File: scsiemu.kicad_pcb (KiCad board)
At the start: 2 copper layers, 65 x 41.7 mm, 38 parts, among them J1 RasPi, J2 SCSI, J3 USB_POWER, J4 POWER 5V, J5 I2C, U1 74LS641-1, U2 74LS641-1, U3 74LS641-1, U4 74LS641-1

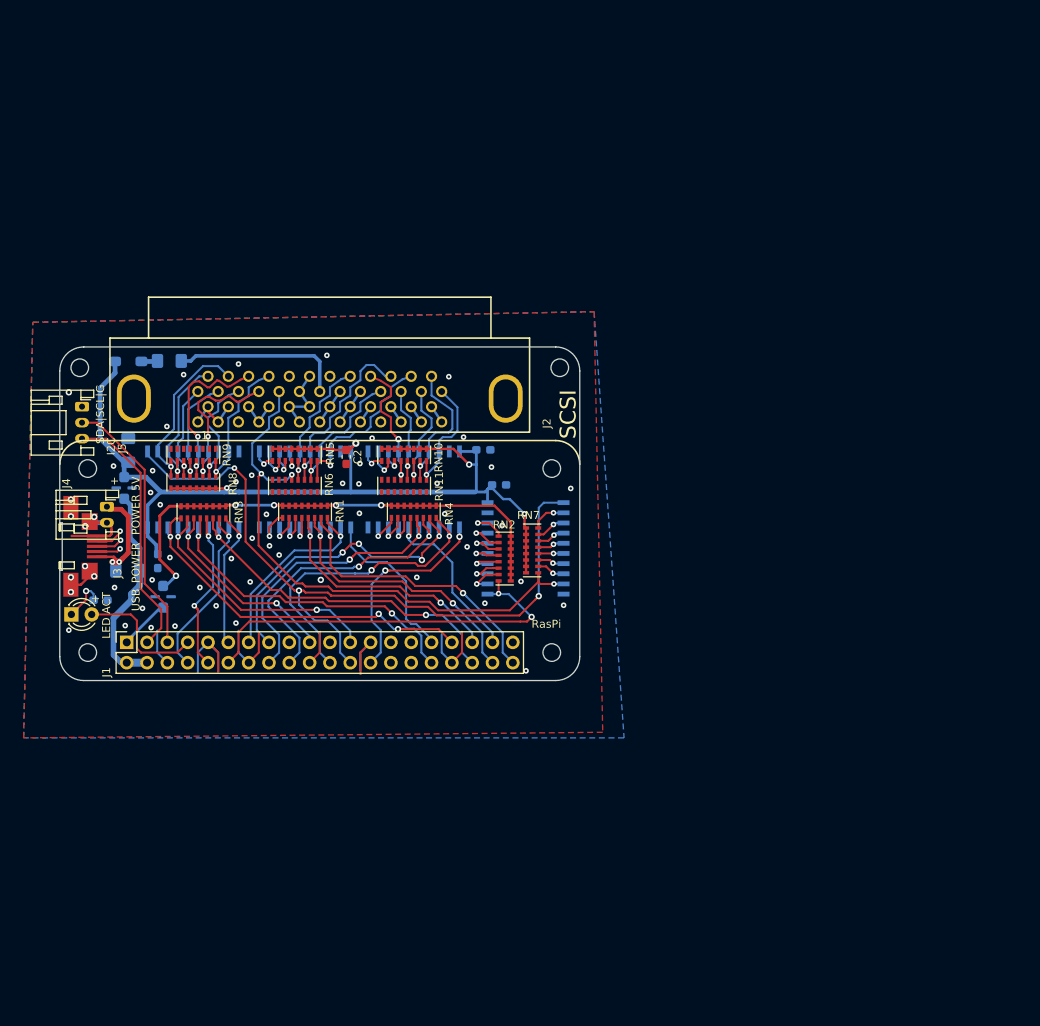
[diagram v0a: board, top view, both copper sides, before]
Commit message: update libs update PCBs update schematic
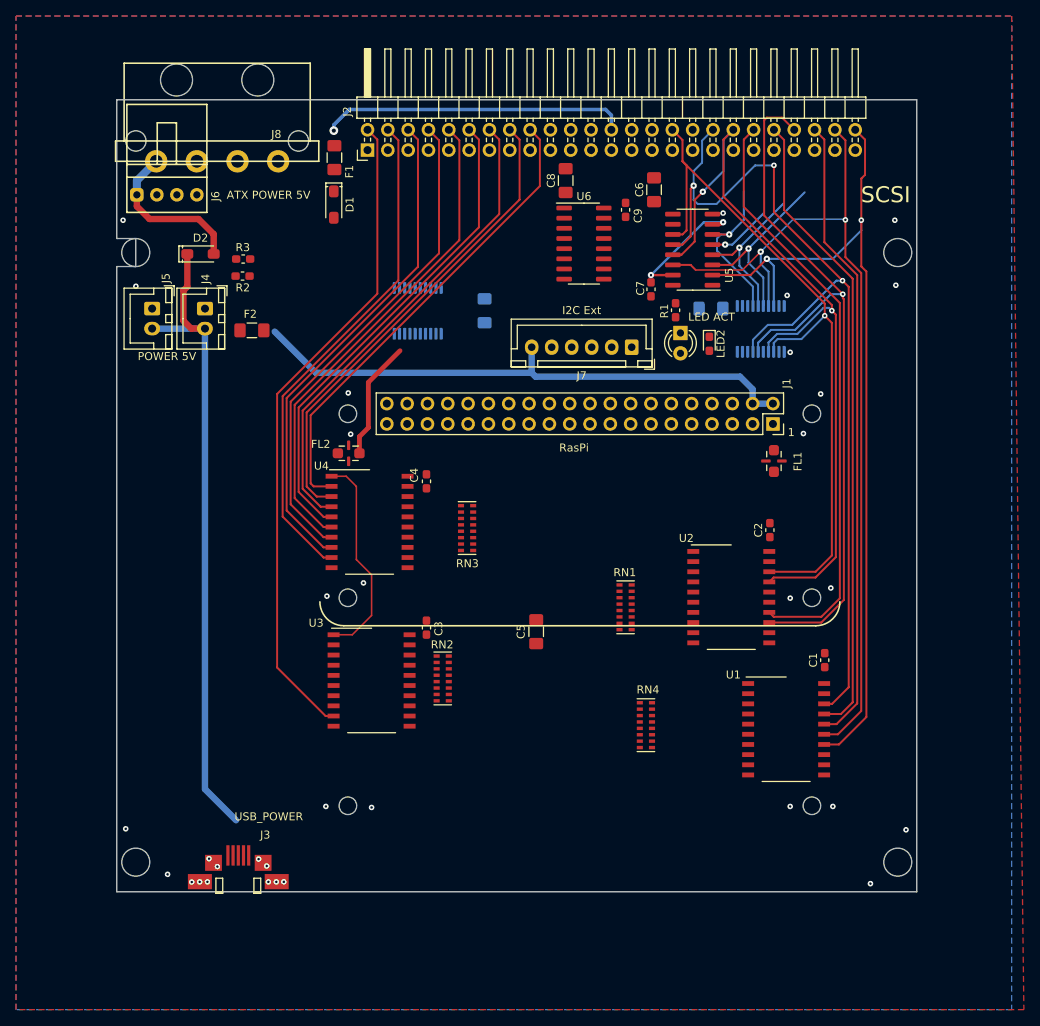
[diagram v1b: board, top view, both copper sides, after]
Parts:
- removed REF** (x6): MountingHole_2.2mm_M2, MountingHole:MountingHole_2.2mm_M2
- removed RN10, RN5, RN7, RN8: 220, Resistor_SMD:R_Cat16-8
- removed RN11, RN6, RN9: 330, Resistor_SMD:R_Cat16-8
- added C10: 10u, Capacitor_SMD:C_1206_3216Metric_Pad1.42x1.75mm_HandSolder, B.Cu at (183.9, 64.0)
- added C11: 10u, Capacitor_SMD:C_1206_3216Metric_Pad1.42x1.75mm_HandSolder, B.Cu at (155.6, 64.3)
- added C6: 10u, Capacitor_SMD:C_1206_3216Metric_Pad1.42x1.75mm_HandSolder, F.Cu at (176.8, 49.1)
- added C7: 2.2u, Capacitor_SMD:C_0603_1608Metric_Pad1.05x0.95mm_HandSolder, F.Cu at (176.4, 61.6)
- added C8: 10u, Capacitor_SMD:C_1206_3216Metric_Pad1.42x1.75mm_HandSolder, F.Cu at (165.7, 48.0)
- added C9: 2.2u, Capacitor_SMD:C_0603_1608Metric_Pad1.05x0.95mm_HandSolder, F.Cu at (173.2, 51.7)
- added D2: SBD, local_lib:D_SOD-123_HandSoldering, F.Cu at (120.1, 57.2)
- added J6: AT Power 5V (171826-4), local_lib:Molex_171826-4, F.Cu at (119.6, 49.8)
- added J7: I2C Ext, Connector_JST:JST_XH_B6B-XH-A_1x06_P2.50mm_Vertical, F.Cu at (174.0, 68.8)
- added J8: AT Power 5V (641737-1), local_lib:TE_641737-1, F.Cu at (122.2, 35.4)
- added LED2: LED ACT, LED_SMD:LED_0603_1608Metric_Pad1.05x0.95mm_HandSolder, F.Cu at (183.7, 68.4)
- added MH1: Raspi Mount, MountingHole:MountingHole_2.2mm_M2, F.Cu at (138.5, 100.2)
- added MH10: Raspi Mount, MountingHole:MountingHole_2.2mm_M2, F.Cu at (138.5, 126.2)
- added MH2: Raspi Mount, MountingHole:MountingHole_2.2mm_M2, F.Cu at (138.5, 77.2)
- added MH3: Raspi Mount, MountingHole:MountingHole_2.2mm_M2, F.Cu at (196.5, 77.2)
- added MH4: Raspi Mount, MountingHole:MountingHole_2.2mm_M2, F.Cu at (196.5, 100.2)
- added MH5: HDD Mount, MountingHole:MountingHole_3.5mm, F.Cu at (112.0, 57.0)
- added MH6: HDD Mount, MountingHole:MountingHole_3.5mm, F.Cu at (112.0, 133.2)
- added MH7: HDD Mount, MountingHole:MountingHole_3.5mm, F.Cu at (207.2, 57.0)
- added MH8: HDD Mount, MountingHole:MountingHole_3.5mm, F.Cu at (207.2, 133.2)
- added MH9: Raspi Mount, MountingHole:MountingHole_2.2mm_M2, F.Cu at (196.5, 126.2)
- added R2: 2.2k, Resistor_SMD:R_0603_1608Metric_Pad1.05x0.95mm_HandSolder, F.Cu at (125.3, 59.9)
- added R3: 2.7k, Resistor_SMD:R_0603_1608Metric_Pad1.05x0.95mm_HandSolder, F.Cu at (125.4, 57.8)
- added U5: DS2105Z, Package_SO:SOIC-16_3.9x9.9mm_P1.27mm, F.Cu at (181.6, 56.6)
- added U6: DS2105Z, Package_SO:SOIC-16_3.9x9.9mm_P1.27mm, F.Cu at (168.0, 55.9)
- added U7: TL2218-285, Package_SO:TSSOP-20_4.4x6.5mm_P0.65mm, B.Cu at (190.1, 66.5)
- added U8: TL2218-285, Package_SO:TSSOP-20_4.4x6.5mm_P0.65mm, B.Cu at (147.2, 64.3)
- C1, C4: value 0.1u JB -> 0.1u; moved to F.Cu
- C2: value 0.1u JB -> 0.1u
- C3: value 0.1u JIS B -> 0.1u; moved to F.Cu
- C5: value 10u JB -> 10u; moved to F.Cu
- D1: footprint cd_device:D_SOD-123_HandSoldering -> local_lib:D_SOD-123_HandSoldering; moved to F.Cu
- F1, FL1, FL2, R1, U1, U2, U3, U4: moved to F.Cu
- F2: value 1A -> 2A; moved to F.Cu
- J2: footprint local_lib:DSUB50P -> Connector_PinHeader_2.54mm:PinHeader_2x25_P2.54mm_Horizontal
- J4: footprint Connector_JST:JST_PH_S2B-PH-K_1x02_P2.00mm_Horizontal -> Connector_JST:JST_XH_B2B-XH-A_1x02_P2.50mm_Vertical
- J5: value I2C -> POWER 5V; footprint Connector_JST:JST_PH_S3B-PH-K_1x03_P2.00mm_Horizontal -> Connector_JST:JST_XH_B2B-XH-A_1x02_P2.50mm_Vertical
- moved J1 85.3 mm to (191.6, 78.4), turned to 270 degrees
- moved LED1 83.9 mm to (180.1, 67.1), turned to 270 degrees
- moved R1 80.5 mm to (179.5, 64.2), turned to 90 degrees
- moved FL1 78.2 mm to (191.8, 83.1), turned to 270 degrees
- moved C5 55.8 mm to (162.1, 104.4), turned to 270 degrees
- moved U1 55.4 mm to (193.3, 116.6), turned to 0 degrees
- moved U2 55.0 mm to (186.4, 100.1), turned to 0 degrees
- moved C2 53.7 mm to (191.3, 91.7), turned to 90 degrees
- moved C1 50.1 mm to (198.1, 108.0), turned to 90 degrees
- moved J3 46.8 mm to (124.8, 135.6), turned to 0 degrees
- moved RN1 41.8 mm to (173.2, 101.3), turned to 180 degrees
- moved RN4 39.4 mm to (175.8, 116.1), turned to 180 degrees
- moved C3 34.6 mm to (148.3, 103.9), turned to 90 degrees
- moved F2 33.8 mm to (126.5, 66.7)
- moved RN3 33.0 mm to (153.4, 91.4), turned to 0 degrees
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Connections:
- D1 pad 2: VCC -> /5V_DC
- F2 pad 1: Net-(F2-Pad1) -> /5V_DC
- F2 pad 2: Net-(F2-Pad2) -> Net-(D2-Pad1)
- FL2 pad 3: Net-(F2-Pad1) -> /5V_DC
- J1 pad 2: Net-(F2-Pad1) -> /5V_DC
- J1 pad 21: Net-(J1-Pad21) -> /AT_POWER_ON
- J1 pad 27: Net-(J1-Pad27) -> /EXT1
- J1 pad 28: Net-(J1-Pad28) -> /EXT2
- J1 pad 4: Net-(F2-Pad1) -> /5V_DC
- J2 pad 10: GND -> /S_D4
- J2 pad 12: GND -> /S_D5
- J2 pad 14: GND -> /S_D6
- J2 pad 16: GND -> /S_D7
- J2 pad 18: GND -> /S_DP
- J2 pad 2: GND -> /S_D0
- J2 pad 25: GND -> Net-(J2-Pad25)
- J2 pad 26: /S_D0 -> Net-(F1-Pad1)
- J2 pad 27: /S_D1 -> GND
- J2 pad 28: /S_D2 -> GND
- J2 pad 29: /S_D3 -> GND
- J2 pad 30: /S_D4 -> GND
- J2 pad 31: /S_D5 -> GND
- J2 pad 32: /S_D6 -> /S_ATN
- J2 pad 33: /S_D7 -> GND
- J2 pad 34: /S_DP -> Net-(J2-Pad34)
- J2 pad 36: GND -> /S_BSY
- J2 pad 38: Net-(F1-Pad1) -> /S_ACK
- J2 pad 4: GND -> /S_D1
- J2 pad 40: GND -> /S_RST
- J2 pad 41: Net-(J2-Pad41) -> GND
- J2 pad 42: GND -> /S_MSG
- J2 pad 43: Net-(J2-Pad43) -> GND
- J2 pad 44: Net-(J2-Pad44) -> /S_SEL
- J2 pad 45: Net-(J2-Pad45) -> GND
- J2 pad 46: Net-(J2-Pad46) -> /S_CD
- J2 pad 47: Net-(J2-Pad47) -> GND
- J2 pad 48: Net-(J2-Pad48) -> /S_REQ
- J2 pad 49: Net-(J2-Pad49) -> GND
- J2 pad 50: Net-(J2-Pad50) -> /S_IO
- J2 pad 6: GND -> /S_D2
- J2 pad 8: GND -> /S_D3
- J3 pad 1: Net-(F2-Pad2) -> Net-(D2-Pad1)
- J4 pad 1: Net-(F2-Pad2) -> GND
- J4 pad 2: GND -> Net-(D2-Pad1)
- J5 pad 2: /I2C_SCL -> Net-(D2-Pad1)
- RN1 pad 3: Net-(RN1-Pad3) -> /SEL
- RN1 pad 4: Net-(RN1-Pad4) -> /RST
- RN1 pad 5: /ATN -> Net-(RN1-Pad5)
- RN1 pad 6: /RST -> Net-(RN1-Pad6)
- RN1 pad 8: /SEL -> /ATN
- RN2 pad 8: /DP -> /D0
- RN3 pad 1: /D3 -> /DP
- RN3 pad 2: /D1 -> /D7
- RN3 pad 3: /D0 -> /D6
- RN3 pad 4: /D2 -> /D5
- RN3 pad 5: /D5 -> /D4
- RN3 pad 6: /D6 -> /D3
- RN3 pad 7: /D4 -> /D2
- RN3 pad 8: /D7 -> /D1
- RN4 pad 4: /BSY -> /IO
- RN4 pad 5: /MSG -> /REQ
- RN4 pad 7: /REQ -> /MSG
- RN4 pad 8: /IO -> /BSY
- U1 pad 14: Net-(J2-Pad43) -> /S_IO
- U1 pad 15: Net-(J2-Pad46) -> /S_REQ
- U1 pad 16: Net-(J2-Pad48) -> /S_CD
- U1 pad 17: Net-(J2-Pad49) -> /S_MSG
- U1 pad 18: Net-(J2-Pad50) -> /S_BSY
- U1 pad 2: /IO -> /BSY
- U1 pad 3: /REQ -> /MSG
- U1 pad 5: /MSG -> /REQ
- U1 pad 6: /BSY -> /IO
- U2 pad 13: Net-(RN5-Pad3) -> /S_SEL
- U2 pad 14: Net-(RN5-Pad4) -> /S_RST
- U2 pad 15: Net-(J2-Pad41) -> Net-(U2-Pad15)
- U2 pad 16: Net-(J2-Pad45) -> Net-(U2-Pad16)
- U2 pad 17: Net-(J2-Pad44) -> /S_ACK
- U2 pad 18: Net-(J2-Pad47) -> /S_ATN
- U2 pad 2: /SEL -> /ATN
- U2 pad 4: /RST -> Net-(RN1-Pad6)
- U2 pad 5: /ATN -> Net-(RN1-Pad5)
- U2 pad 6: Net-(RN1-Pad4) -> /RST
- U2 pad 7: Net-(RN1-Pad3) -> /SEL
- U3 pad 11: /DP -> /D0
- U3 pad 9: /S_DP -> /S_D0
- U4 pad 11: /D7 -> /D1
- U4 pad 12: /D4 -> /D2
- U4 pad 13: /D6 -> /D3
- U4 pad 14: /D5 -> /D4
- U4 pad 15: /D2 -> /D5
- U4 pad 16: /D0 -> /D6
- U4 pad 17: /D1 -> /D7
- U4 pad 18: /D3 -> /DP
- U4 pad 2: /S_D3 -> /S_DP
- U4 pad 3: /S_D1 -> /S_D7
- U4 pad 4: /S_D0 -> /S_D6
- U4 pad 5: /S_D2 -> /S_D5
- U4 pad 6: /S_D5 -> /S_D4
- U4 pad 7: /S_D6 -> /S_D3
- U4 pad 8: /S_D4 -> /S_D2
- U4 pad 9: /S_D7 -> /S_D1
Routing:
- net /S_BSY: track 0.00 -> 120.0 mm, vias 0 -> 3
- net VCC: track 132.8 -> 14.9 mm, vias 4 -> 0
- net /S_REQ: track 0.00 -> 111.5 mm, vias 0 -> 2
- net /S_IO: track 0.00 -> 109.5 mm, vias 0 -> 2
- net /S_CD: track 0.00 -> 102.4 mm, vias 0 -> 1
- net /S_SEL: track 0.00 -> 101.5 mm, vias 0 -> 2
- net GND: track 100.9 -> 0.00 mm, vias 55 -> 33
- net /S_ACK: track 0.00 -> 99.8 mm, vias 0 -> 2
- net /S_MSG: track 0.00 -> 99.7 mm, vias 0 -> 1
- net /S_RST: track 0.00 -> 94.3 mm, vias 0 -> 1
- net /S_ATN: track 0.00 -> 89.8 mm, vias 0 -> 1
- net Net-(D2-Pad1): track 0.00 -> 81.3 mm
- net /5V_DC: track 0.00 -> 70.3 mm
- net /S_D0: track 12.7 -> 82.5 mm, vias 1 -> 0
- net /DTD: track 91.3 -> 26.3 mm, vias 3 -> 0
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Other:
- board size 65 x 41.7 mm -> 100 x 99 mm
- net class Default: clearance 0.2 -> 0.25; via_drill 0.4 -> 0.3
- net class LV added: clearance 0.2, trace_width 0.2, via_dia 0.7, via_drill 0.3
- rule trace_clearance: 0.2 -> 0.25
- board text added: "ATX POWER 5V"
- board text removed: "*"
- board text removed: "+"
- board text removed: "D+"
- board text removed: "D-"
- board text removed: "GND"
- board text removed: "ID"
- board text removed: "SDA|SCL|G"
